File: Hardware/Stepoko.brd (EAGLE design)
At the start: 150 x 80 mm, 173 parts, among them J1 AVR ISP, Q1 16MHZ, Q2 100A/100V, U1 ATMEGA328, U2 CY7C65213, U3 74LVC1G04, U4 LM25011, U5 DRV8811, U6 74HC7014D, U7 74AHC1G08, U8 DRV8811, U9 DRV8811

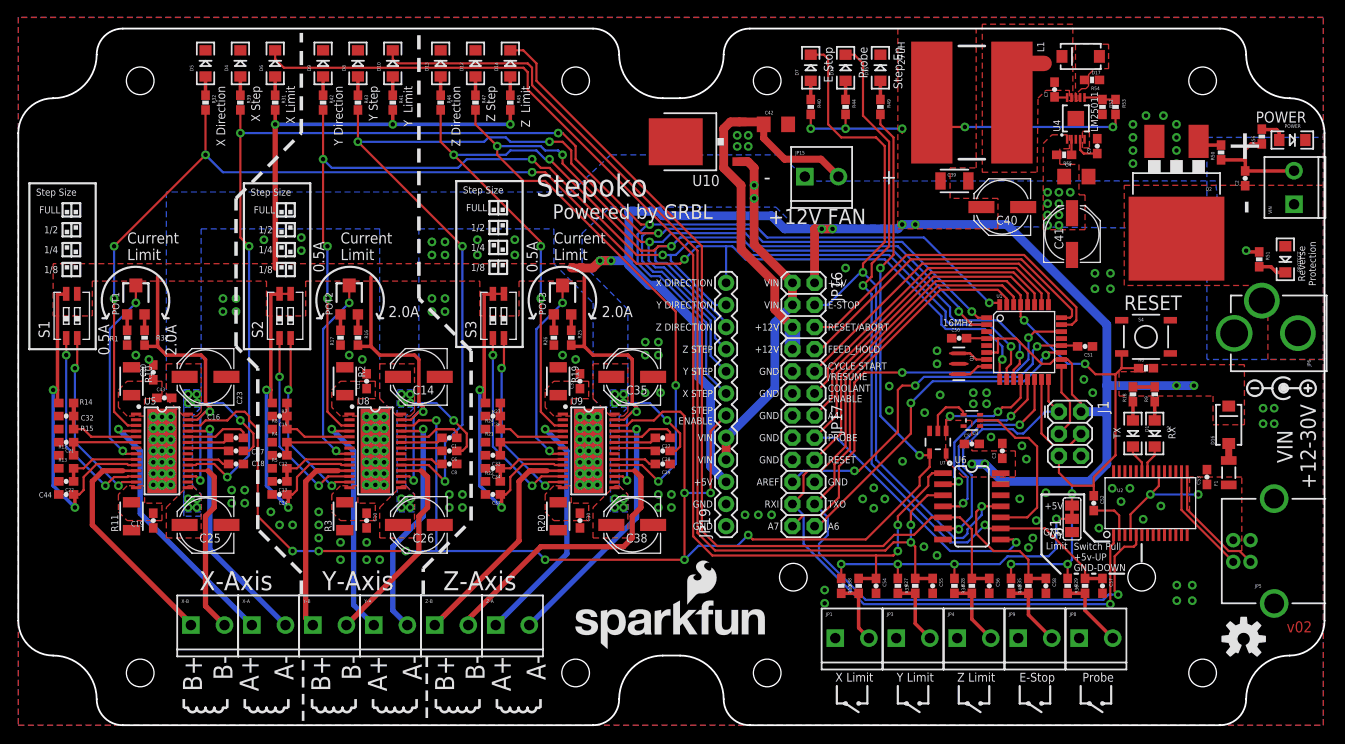
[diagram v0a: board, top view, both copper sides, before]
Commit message: made changes from design review
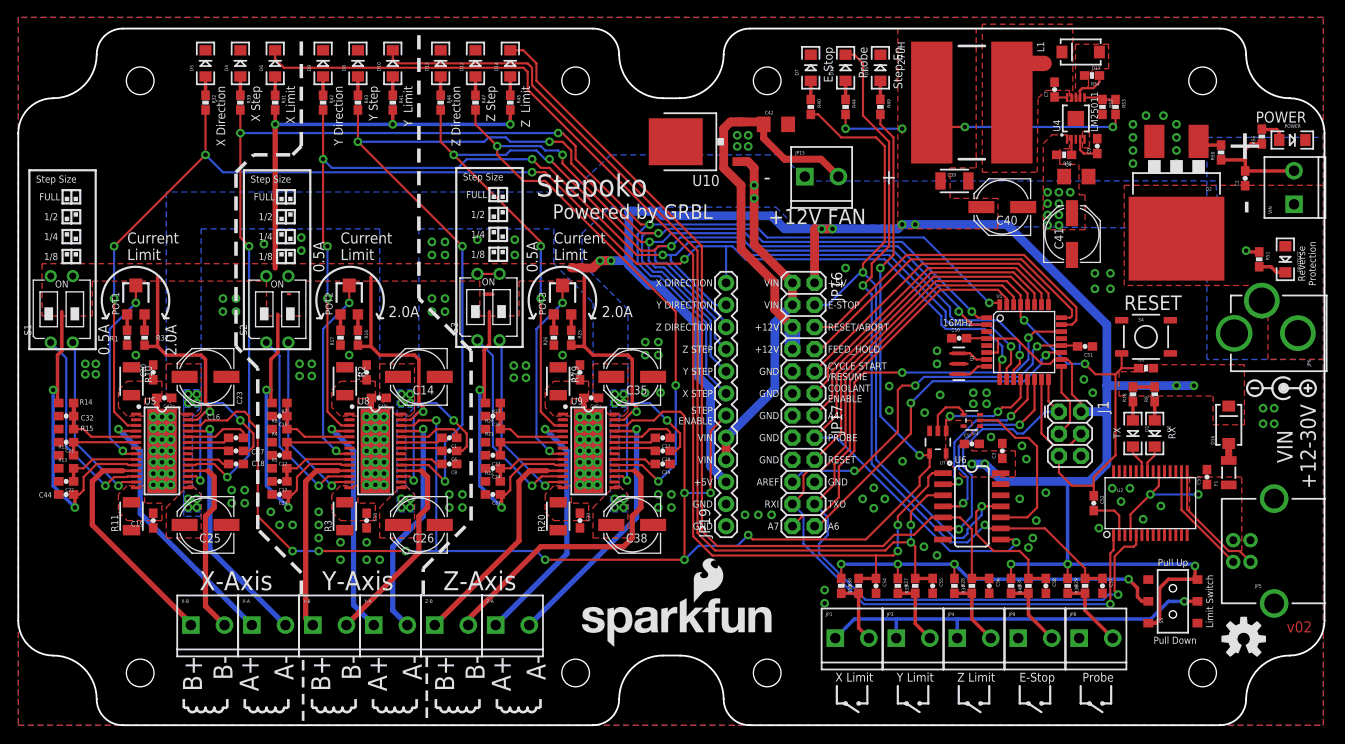
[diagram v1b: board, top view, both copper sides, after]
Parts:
- removed SJ1: Limit Pull Direction, SparkFun-Passives:PAD-JUMPER-3-2OF3_NC_BY_TRACE_YES_SILK_LARGE
- removed U$3: (no value), SparkFun-Boards:FLANGED_RED_ENCLOSURE-OUTLINE
- added C45, C46: 0.1uF, SparkFun-Capacitors:0603-CAP
- added S5: DPDT, SparkFun-Electromechanical:AYZ0202
- added U$1: (no value), SparkFun-Boards:FLANGED_RED_ENCLOSURE-DIMENSION-NO-INNER-HOLES
- C43: value 1000pF -> 0.1uF
- S1, S2, S3: value 2-POS-DIP -> 2-POS-DIPCTS-THRU-HOLE; device SparkFun-Electromechanical:CHS-02A -> SparkFun-Electromechanical:209-2LPST
- moved S3 1.14 mm to (54.0, 48.0)
- moved C11 1.02 mm to (40.0, 40.5)
- moved C31 1.02 mm to (64.5, 40.5)
- moved S1 0.92 mm to (4.99, 47.8)
- moved S2 0.80 mm to (29.7, 47.8)
- moved LOGO2 0.80 mm to (64.0, 8.89)
- moved D17 0.51 mm to (122.0, 77.3)
- moved R54 0.51 mm to (123.3, 74.6)
- turned C43 to 180 degrees
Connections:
- new net N$4: JP1.1, JP3.1, JP4.1, S5.5
- net 5V: now also S5.1, S5.6; no longer R40.2, SJ1.3
- net ESTOP: now also R40.2; no longer D7.C
- net GND: now also C43.2, C45.2, C46.2, D7.C, S5.3, S5.4; no longer JP1.1, JP3.1, JP4.1, SJ1.1
- net N$95: now also S5.2; no longer SJ1.2
- net VIN: now also C43.1, C45.1, C46.1
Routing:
- net N$4: track 0.00 -> 47.7 mm, vias 0 -> 1
- net 5V: track 521.0 -> 532.5 mm, vias 33 -> 32
- net ESTOP: track 97.2 -> 90.0 mm
- net N$95: track 35.6 -> 42.6 mm
- net N$1: track 0.00 -> 4.19 mm
- net GND: track 0.00 -> 3.39 mm, vias 119 -> 123
- net N$15: track 21.3 -> 20.7 mm, vias 2 -> 1
- net N$34: track 21.3 -> 20.8 mm, vias 2 -> 1
- net N$77: track 22.8 -> 23.3 mm, vias 2 -> 1
- net N$76: track 21.3 -> 21.1 mm, vias 2 -> 1
- net N$35: track 22.8 -> 23.0 mm, vias 2 -> 1
- net N$23: track 22.8 -> 22.9 mm, vias 2 -> 1
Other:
- board text added: "Limit Switch"
- board text added: "Pull Down"
- board text added: "Pull Up"
- board text removed: "Limit"
- board text removed: "Switch Pull +5v-UP GND-DOWN"
